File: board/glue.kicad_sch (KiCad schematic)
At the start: 14 parts, among them J1 Conn_01x05_Pin, J8 CF Card, U12 GLUE

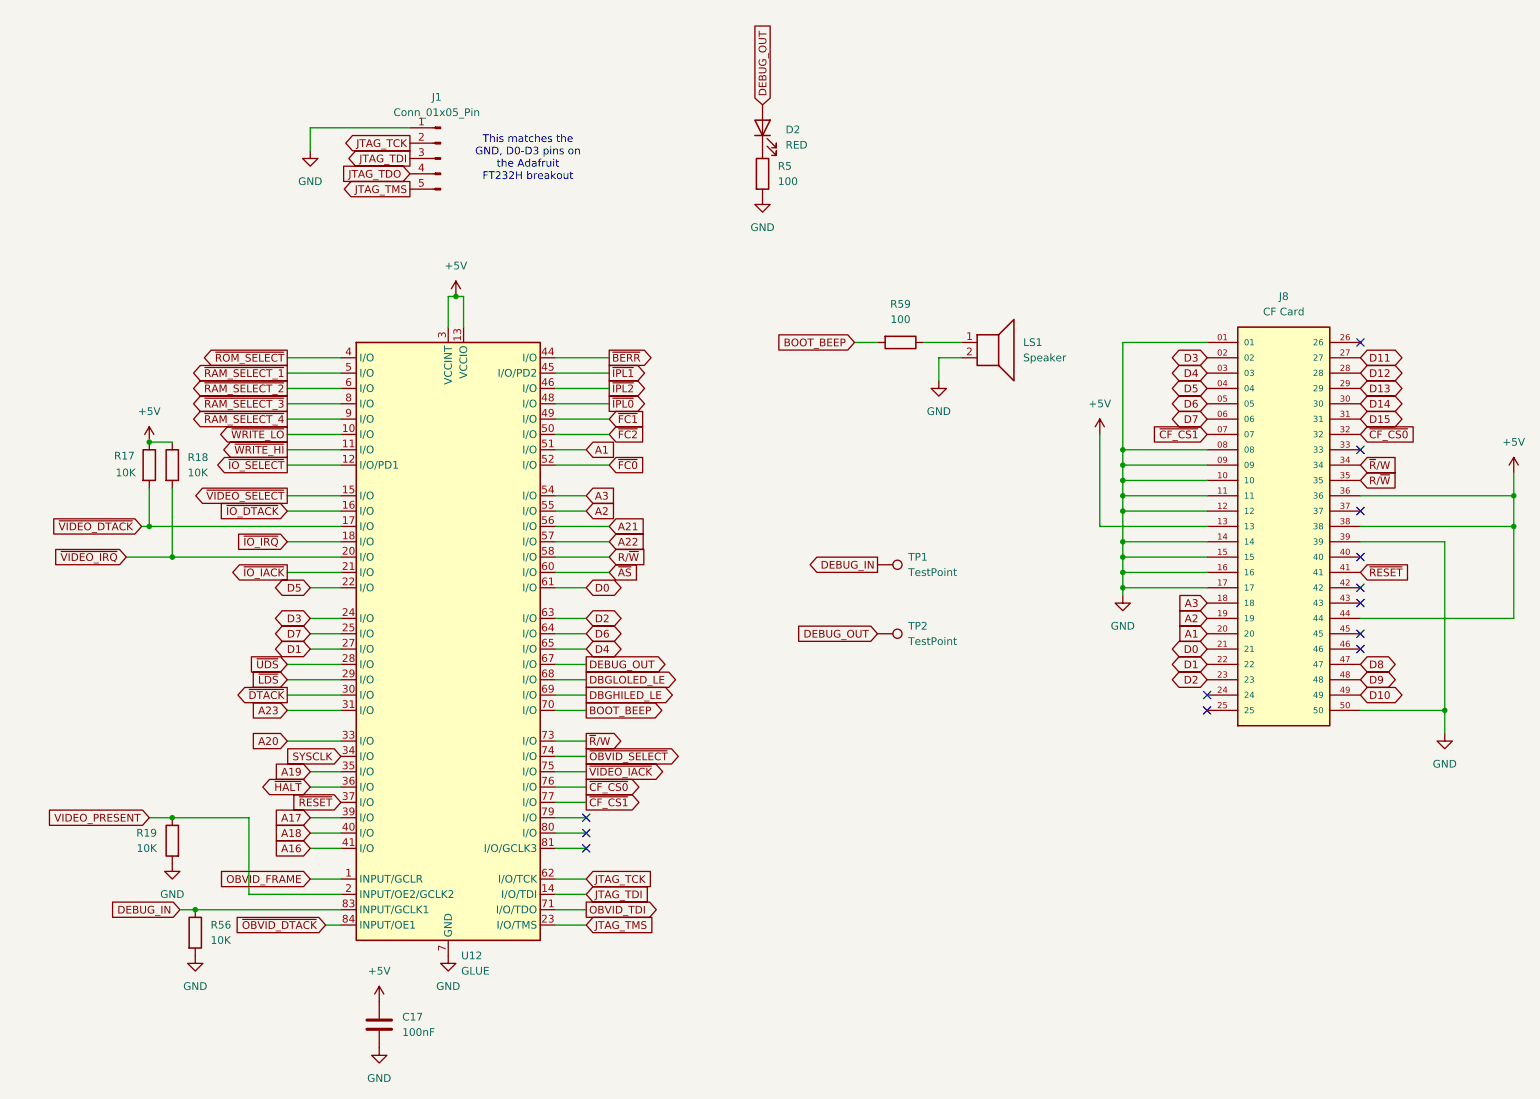
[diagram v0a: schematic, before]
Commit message: checkpoint
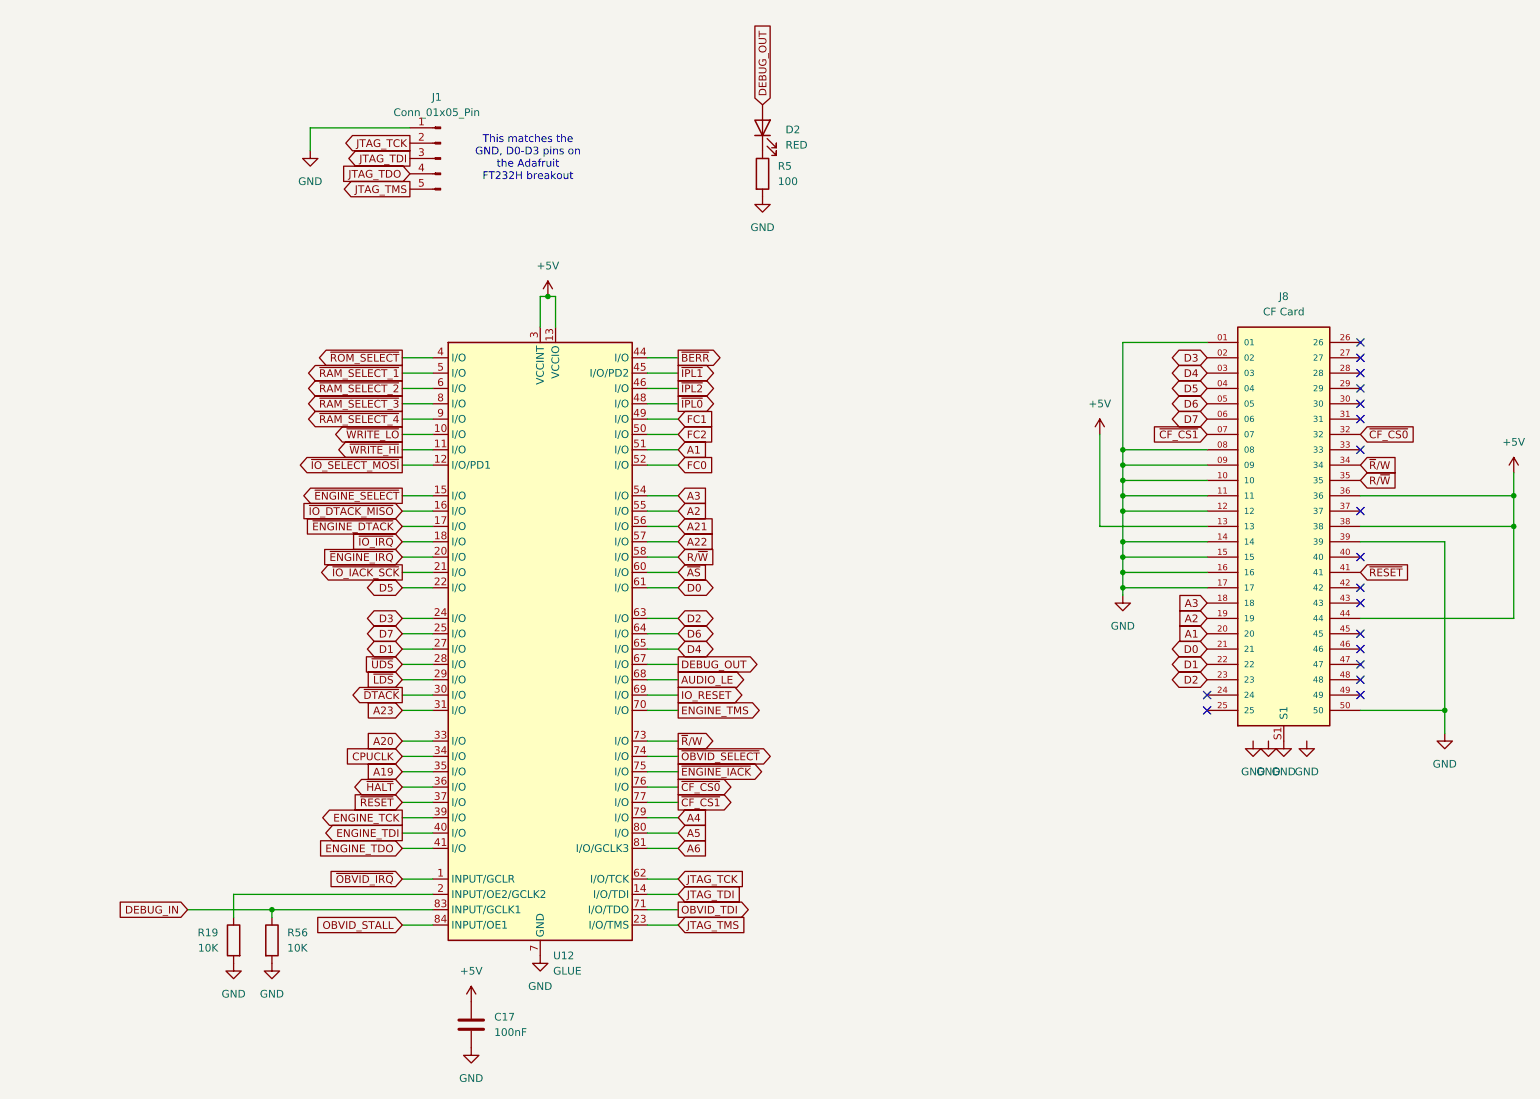
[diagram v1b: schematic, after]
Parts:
- removed LS1: Speaker, Buzzer_Beeper:MagneticBuzzer_StarMicronics_QMX, symbol Device:Speaker
- removed R17, R18: 10K, Resistor_THT:R_Axial_DIN0207_L6.3mm_D2.5mm_P10.16mm_Horizontal, symbol Device:R
- removed R59: 100, Resistor_THT:R_Axial_DIN0207_L6.3mm_D2.5mm_P10.16mm_Horizontal, symbol Device:R
- removed TP1, TP2: TestPoint, Connector_PinHeader_2.54mm:PinHeader_1x01_P2.54mm_Vertical, symbol Connector:TestPoint
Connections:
- net GND: now also J8.S1, J8.S2, J8.S3, J8.S4
- net A4: now reaches U12.79 (I/O)
- net A5: now reaches U12.80 (I/O)
- net A6: now reaches U12.81 (I/O/GCLK3)
- net A16 renamed ENGINE_TDO
- net A17 renamed ENGINE_TCK
- net A18 renamed ENGINE_TDI
- net BOOT_BEEP renamed ENGINE_TMS
- net D10: no longer names the net of J8.49
- net D11: no longer names the net of J8.27
- net D12: no longer names the net of J8.28
- net D13: no longer names the net of J8.29
- net D14: no longer names the net of J8.30
- net D15: no longer names the net of J8.31
- net D8: no longer names the net of J8.47
- net D9: no longer names the net of J8.48
- net DBGHILED_LE renamed IO_RESET
- net DBGLOLED_LE renamed AUDIO_LE
- net OBVID_FRAME renamed ~{OBVID_IRQ}
- net SYSCLK renamed CPUCLK
- net VIDEO_PRESENT: no longer names the net of R19.1, U12.2 (INPUT/OE2/GCLK2)
- net ~{FC0} renamed FC0
- net ~{FC1} renamed FC1
- net ~{FC2} renamed FC2
- net ~{IO_DTACK} renamed ~{IO_DTACK_MISO}
- net ~{IO_IACK} renamed ~{IO_IACK_SCK}
- net ~{IO_SELECT} renamed ~{IO_SELECT_MOSI}
- net ~{OBVID_DTACK} renamed OBVID_STALL
- net ~{VIDEO_DTACK} renamed ~{ENGINE_DTACK}
- net ~{VIDEO_IACK} renamed ~{ENGINE_IACK}
- net ~{VIDEO_IRQ} renamed ~{ENGINE_IRQ}
- net ~{VIDEO_SELECT} renamed ~{ENGINE_SELECT}
- no-connect marks 13 -> 18
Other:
- moved on the sheet: C17, R19, R56, U12

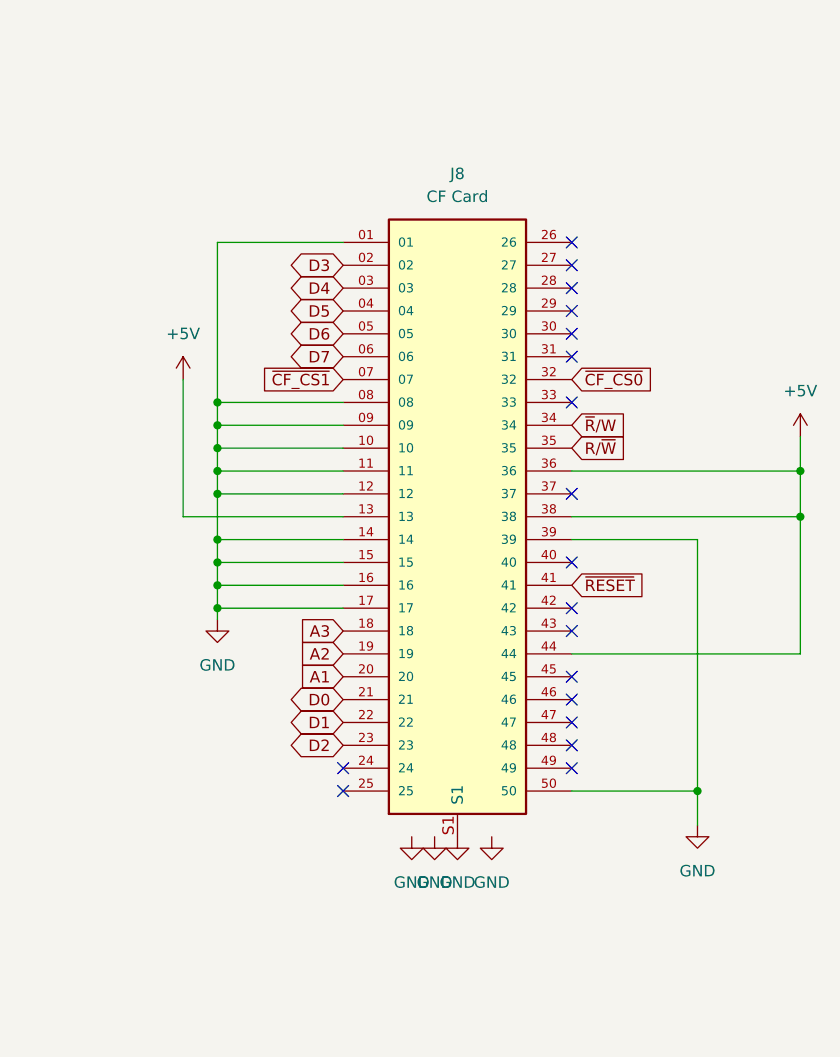
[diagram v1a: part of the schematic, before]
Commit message: Board rev1 PCB complete, already have a spot fix
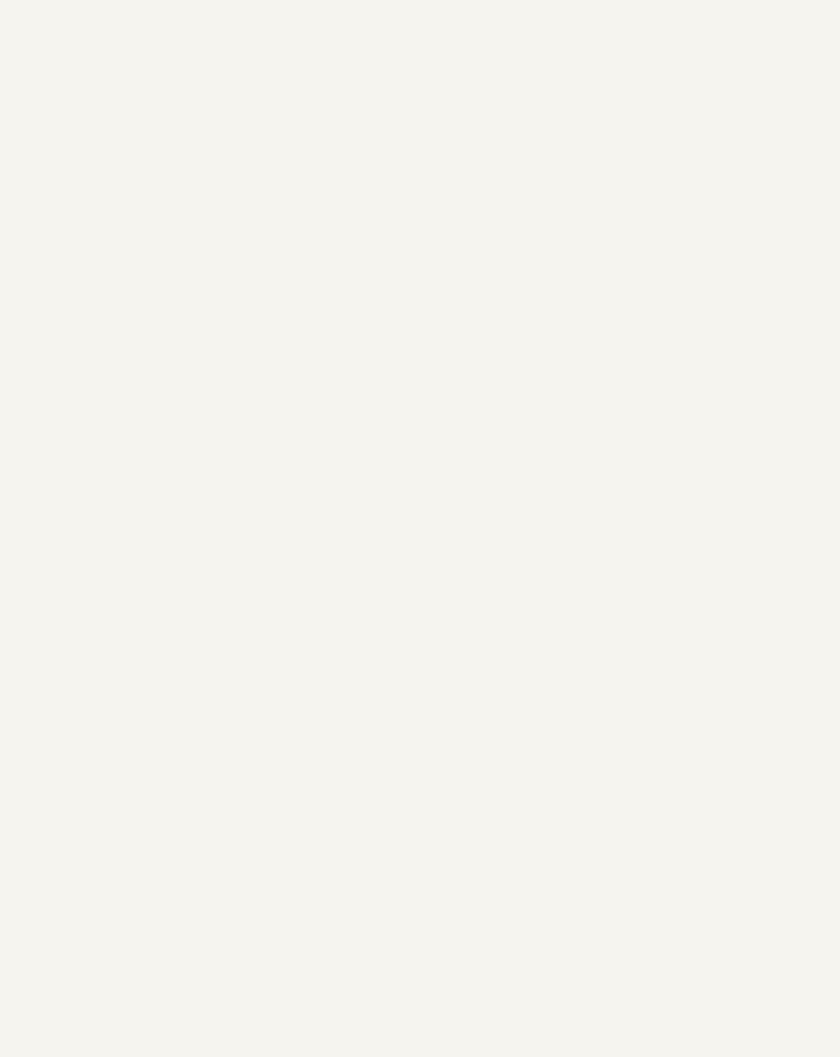
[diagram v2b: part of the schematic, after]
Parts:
- removed J8: CF Card, board:SAMTEC_CFT-125-01-L-D-RA-01-SL, symbol SAMTEC:CFT-125-01-L-D-RA-01-SL
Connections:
- no-connect marks 18 -> 0
